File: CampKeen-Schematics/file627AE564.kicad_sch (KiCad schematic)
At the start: 23 parts, among them Q26 2N7000, Q27 2N7000, Q28 2N7000, Q29 2N7000, Q54 LTV-847

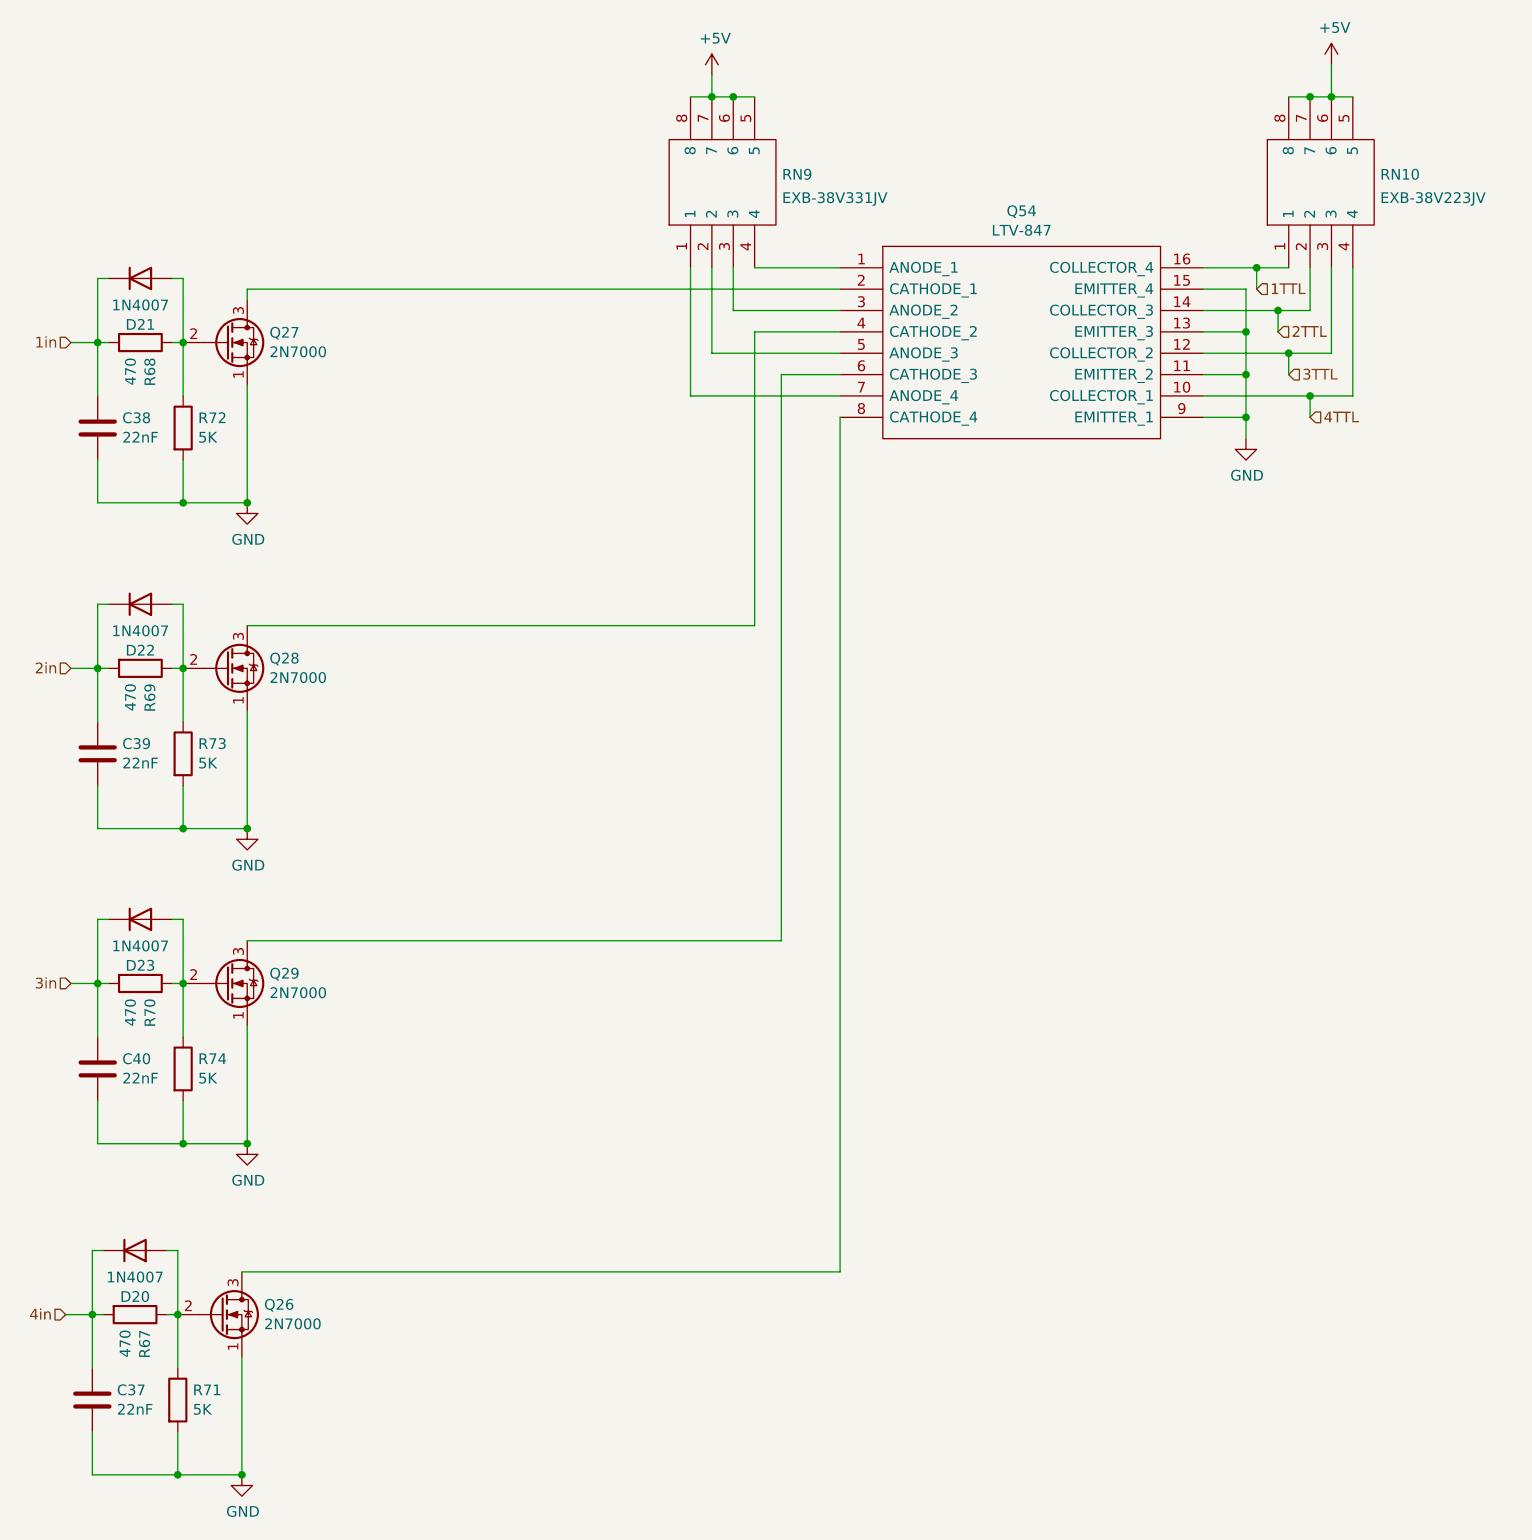
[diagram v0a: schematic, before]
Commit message: working on getting the board cleaned enough to start placing the new designs and chips.
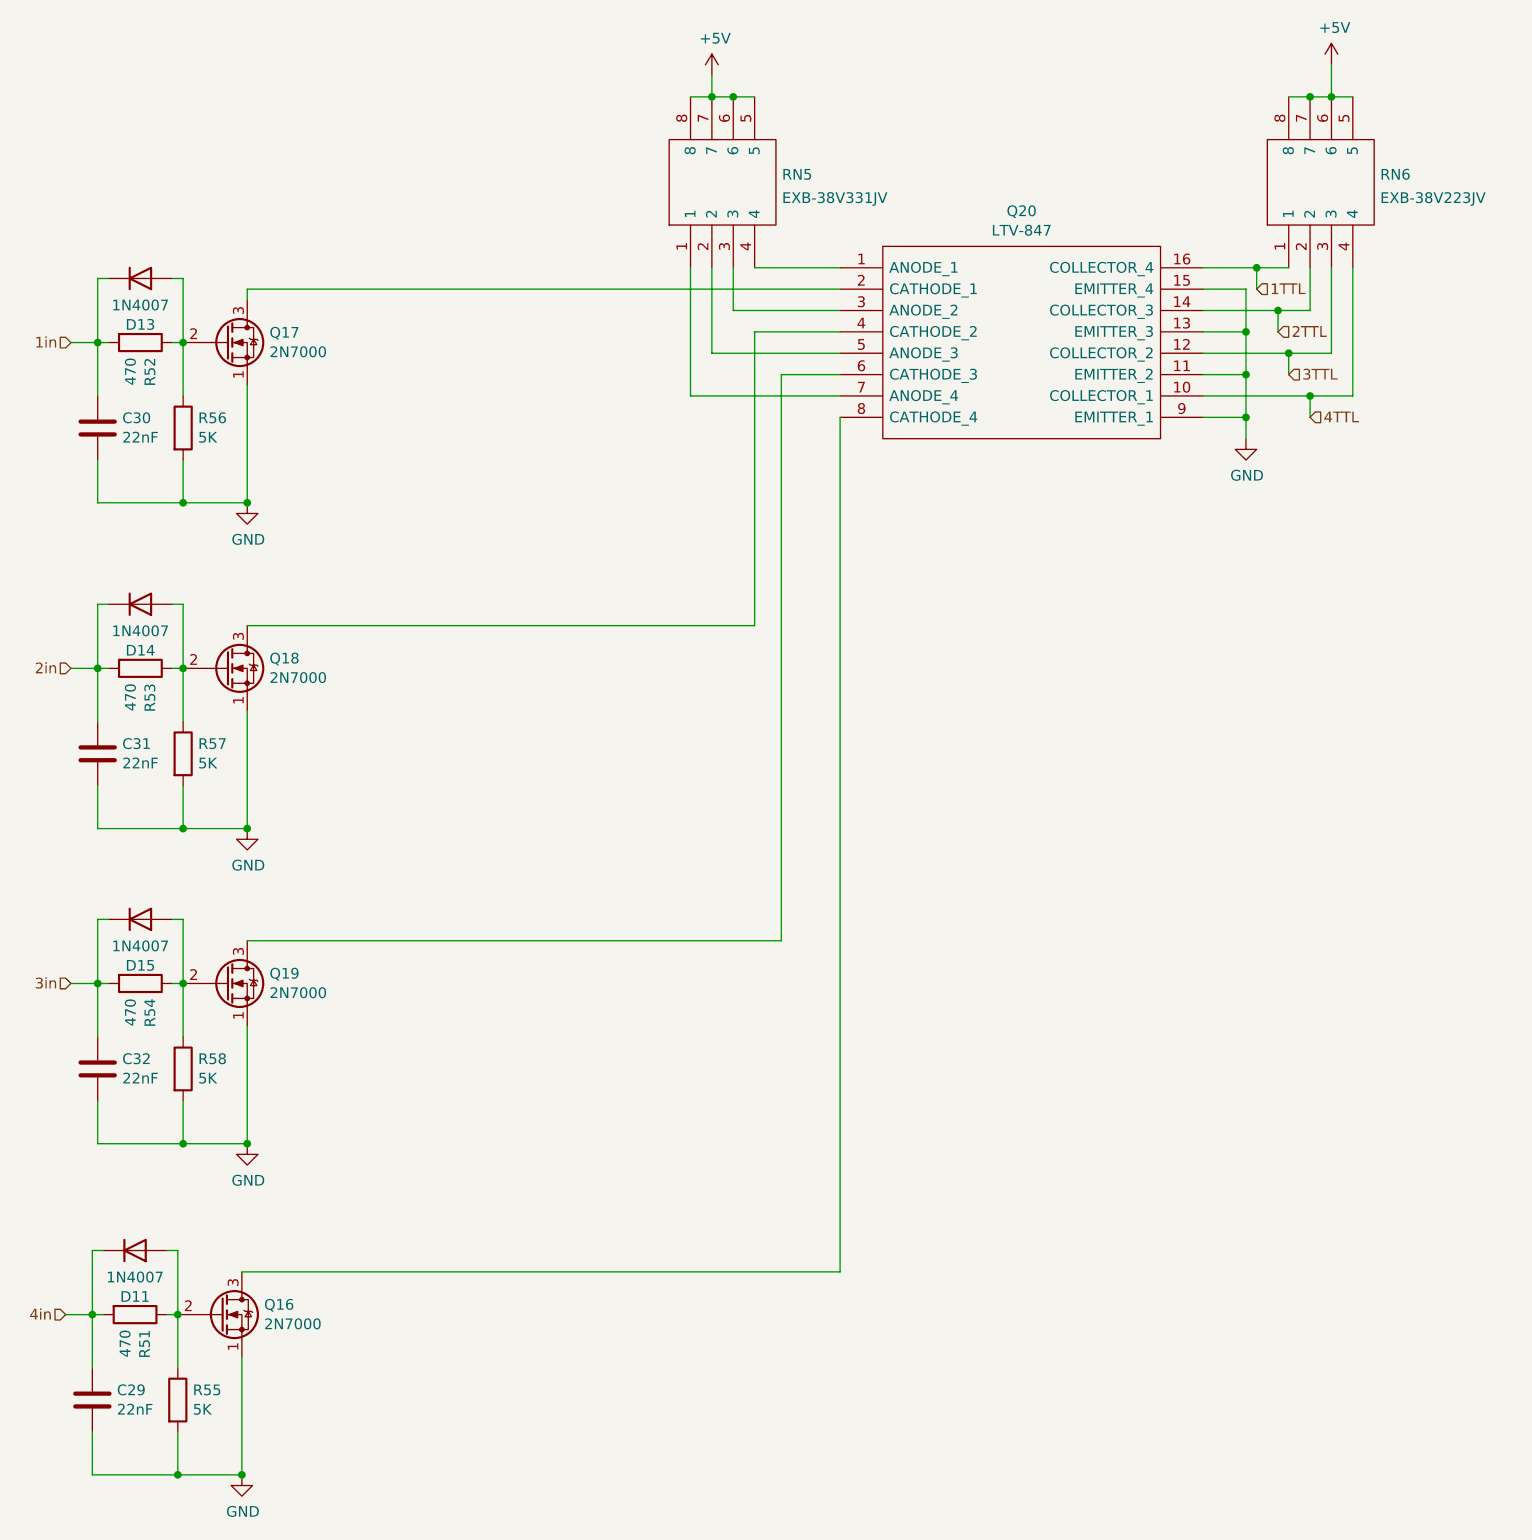
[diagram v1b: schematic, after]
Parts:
- renumbered C37 to C29, C38 to C30, C39 to C31, C40 to C32, D20 to D11, D21 to D13, D22 to D14, D23 to D15, Q26 to Q16, Q27 to Q17, Q28 to Q18, Q29 to Q19, Q54 to Q20, R67 to R51, R68 to R52, R69 to R53, R70 to R54, R71 to R55, R72 to R56, R73 to R57, R74 to R58, RN9 to RN5, RN10 to RN6
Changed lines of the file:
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@@
   (symbol (lib_id "Device:R") (at 67.945 132.08 270)
     (in_bom yes) (on_board yes)
-    (property "Reference" "R70" (id 0) (at 69.1134 133.858 0)
+    (property "Reference" "R54" (id 0) (at 69.1134 133.858 0)
       (effects (font (size 1.27 1.27)) (justify left))
     )
@@
   (symbol (lib_id "Diode:1N4007") (at 67.945 86.995 0) (mirror x)
     (in_bom yes) (on_board yes)
-    (property "Reference" "D22" (id 0) (at 67.945 92.5068 0))
+    (property "Reference" "D14" (id 0) (at 67.945 92.5068 0))
     (property "Value" "1N4007" (id 1) (at 67.945 90.1954 0))
     (property "Footprint" "Diode_THT:D_DO-41_SOD81_P10.16mm_Horizontal" (id 2) (at 67.945 82.55 0)
@@
   (symbol (lib_id "power:+5V") (at 135.89 24.13 0)
     (in_bom yes) (on_board yes)
-    (property "Reference" "#PWR0152" (id 0) (at 135.89 27.94 0)
+    (property "Reference" "#PWR0111" (id 0) (at 135.89 27.94 0)
       (effects (font (size 1.27 1.27)) hide)
     )
@@
   (symbol (lib_id "Samac_Sys:EXB-38V331JV") (at 133.35 46.99 90)
     (in_bom yes) (on_board yes) (fields_autoplaced)
-    (property "Reference" "RN9" (id 0) (at 144.2212 35.9215 90)
+    (property "Reference" "RN5" (id 0) (at 144.2212 35.9215 90)
       (effects (font (size 1.27 1.27)) (justify right))
     )
@@
   (symbol (lib_id "power:GND") (at 80.645 151.13 0)
     (in_bom yes) (on_board yes)
-    (property "Reference" "#PWR0156" (id 0) (at 80.645 157.48 0)
+    (property "Reference" "#PWR0114" (id 0) (at 80.645 157.48 0)
       (effects (font (size 1.27 1.27)) hide)
     )
@@
   (symbol (lib_id "Transistor_FET:2N7000") (at 78.105 55.88 0)
     (in_bom yes) (on_board yes)
-    (property "Reference" "Q27" (id 0) (at 83.2866 54.7116 0)
+    (property "Reference" "Q17" (id 0) (at 83.2866 54.7116 0)
       (effects (font (size 1.27 1.27)) (justify left))
     )
@@
   (symbol (lib_id "Device:R") (at 67.945 55.88 270)
     (in_bom yes) (on_board yes)
-    (property "Reference" "R68" (id 0) (at 69.1134 57.658 0)
+    (property "Reference" "R52" (id 0) (at 69.1134 57.658 0)
       (effects (font (size 1.27 1.27)) (justify left))
     )
@@
   (symbol (lib_id "Diode:1N4007") (at 67.945 124.46 0) (mirror x)
     (in_bom yes) (on_board yes)
-    (property "Reference" "D23" (id 0) (at 67.945 129.9718 0))
+    (property "Reference" "D15" (id 0) (at 67.945 129.9718 0))
     (property "Value" "1N4007" (id 1) (at 67.945 127.6604 0))
     (property "Footprint" "Diode_THT:D_DO-41_SOD81_P10.16mm_Horizontal" (id 2) (at 67.945 120.015 0)
@@
   (symbol (lib_id "power:GND") (at 199.39 67.31 0)
     (in_bom yes) (on_board yes)
-    (property "Reference" "#PWR0155" (id 0) (at 199.39 73.66 0)
+    (property "Reference" "#PWR0113" (id 0) (at 199.39 73.66 0)
       (effects (font (size 1.27 1.27)) hide)
     )
@@
   (symbol (lib_id "SamacSys_Parts:LTV-847") (at 151.13 46.99 0)
     (in_bom yes) (on_board yes)
-    (property "Reference" "Q54" (id 0) (at 172.72 40.259 0))
+    (property "Reference" "Q20" (id 0) (at 172.72 40.259 0))
     (property "Value" "LTV-847" (id 1) (at 172.72 42.5704 0))
     (property "Footprint" "SamacSys_Parts:DIP762W60P254L1984H450Q16N" (id 2) (at 190.5 44.45 0)
@@
   (symbol (lib_id "power:GND") (at 80.645 113.665 0)
     (in_bom yes) (on_board yes)
-    (property "Reference" "#PWR0123" (id 0) (at 80.645 120.015 0)
+    (property "Reference" "#PWR0108" (id 0) (at 80.645 120.015 0)
       (effects (font (size 1.27 1.27)) hide)
     )
@@
   (symbol (lib_id "power:GND") (at 80.01 190.5 0)
     (in_bom yes) (on_board yes)
-    (property "Reference" "#PWR0150" (id 0) (at 80.01 196.85 0)
+    (property "Reference" "#PWR0110" (id 0) (at 80.01 196.85 0)
       (effects (font (size 1.27 1.27)) hide)
     )
@@
   (symbol (lib_id "Device:R") (at 67.945 94.615 270)
     (in_bom yes) (on_board yes)
-    (property "Reference" "R69" (id 0) (at 69.1134 96.393 0)
+    (property "Reference" "R53" (id 0) (at 69.1134 96.393 0)
       (effects (font (size 1.27 1.27)) (justify left))
     )
@@
   (symbol (lib_id "Diode:1N4007") (at 67.31 163.83 0) (mirror x)
     (in_bom yes) (on_board yes)
-    (property "Reference" "D20" (id 0) (at 67.31 169.3418 0))
+    (property "Reference" "D11" (id 0) (at 67.31 169.3418 0))
     (property "Value" "1N4007" (id 1) (at 67.31 167.0304 0))
     (property "Footprint" "Diode_THT:D_DO-41_SOD81_P10.16mm_Horizontal" (id 2) (at 67.31 159.385 0)
@@
   (symbol (lib_id "Device:R") (at 67.31 171.45 270)
     (in_bom yes) (on_board yes)
-    (property "Reference" "R67" (id 0) (at 68.4784 173.228 0)
+    (property "Reference" "R51" (id 0) (at 68.4784 173.228 0)
       (effects (font (size 1.27 1.27)) (justify left))
     )
@@
   (symbol (lib_id "Device:R") (at 73.025 104.775 0)
     (in_bom yes) (on_board yes)
-    (property "Reference" "R73" (id 0) (at 74.803 103.6066 0)
+    (property "Reference" "R57" (id 0) (at 74.803 103.6066 0)
       (effects (font (size 1.27 1.27)) (justify left))
     )
@@
   (symbol (lib_id "Device:R") (at 73.025 142.24 0)
     (in_bom yes) (on_board yes)
-    (property "Reference" "R74" (id 0) (at 74.803 141.0716 0)
+    (property "Reference" "R58" (id 0) (at 74.803 141.0716 0)
       (effects (font (size 1.27 1.27)) (justify left))
     )
@@
   (symbol (lib_id "Transistor_FET:2N7000") (at 77.47 171.45 0)
     (in_bom yes) (on_board yes)
-    (property "Reference" "Q26" (id 0) (at 82.6516 170.2816 0)
+    (property "Reference" "Q16" (id 0) (at 82.6516 170.2816 0)
       (effects (font (size 1.27 1.27)) (justify left))
     )
@@
   (symbol (lib_id "Device:C") (at 62.865 66.04 0)
     (in_bom yes) (on_board yes)
-    (property "Reference" "C38" (id 0) (at 65.786 64.8716 0)
+    (property "Reference" "C30" (id 0) (at 65.786 64.8716 0)
       (effects (font (size 1.27 1.27)) (justify left))
     )
@@
   (symbol (lib_id "power:GND") (at 80.645 74.93 0)
     (in_bom yes) (on_board yes)
-    (property "Reference" "#PWR0124" (id 0) (at 80.645 81.28 0)
+    (property "Reference" "#PWR0109" (id 0) (at 80.645 81.28 0)
       (effects (font (size 1.27 1.27)) hide)
     )
@@
   (symbol (lib_id "Device:R") (at 73.025 66.04 0)
     (in_bom yes) (on_board yes)
-    (property "Reference" "R72" (id 0) (at 74.803 64.8716 0)
+    (property "Reference" "R56" (id 0) (at 74.803 64.8716 0)
       (effects (font (size 1.27 1.27)) (justify left))
     )
@@
   (symbol (lib_id "Device:R") (at 72.39 181.61 0)
     (in_bom yes) (on_board yes)
-    (property "Reference" "R71" (id 0) (at 74.168 180.4416 0)
+    (property "Reference" "R55" (id 0) (at 74.168 180.4416 0)
       (effects (font (size 1.27 1.27)) (justify left))
     )
@@
   (symbol (lib_id "Transistor_FET:2N7000") (at 78.105 132.08 0)
     (in_bom yes) (on_board yes)
-    (property "Reference" "Q29" (id 0) (at 83.2866 130.9116 0)
+    (property "Reference" "Q19" (id 0) (at 83.2866 130.9116 0)
       (effects (font (size 1.27 1.27)) (justify left))
     )
@@
   (symbol (lib_id "Device:C") (at 62.865 104.775 0)
     (in_bom yes) (on_board yes)
-    (property "Reference" "C39" (id 0) (at 65.786 103.6066 0)
+    (property "Reference" "C31" (id 0) (at 65.786 103.6066 0)
       (effects (font (size 1.27 1.27)) (justify left))
     )
@@
   (symbol (lib_id "power:+5V") (at 209.55 22.86 0)
     (in_bom yes) (on_board yes)
-    (property "Reference" "#PWR0153" (id 0) (at 209.55 26.67 0)
+    (property "Reference" "#PWR0112" (id 0) (at 209.55 26.67 0)
       (effects (font (size 1.27 1.27)) hide)
     )
@@
   (symbol (lib_id "Samac_Sys:EXB-38V223JV") (at 204.47 46.99 90)
     (in_bom yes) (on_board yes) (fields_autoplaced)
-    (property "Reference" "RN10" (id 0) (at 215.3412 35.9215 90)
+    (property "Reference" "RN6" (id 0) (at 215.3412 35.9215 90)
       (effects (font (size 1.27 1.27)) (justify right))
     )
@@
   (symbol (lib_id "Transistor_FET:2N7000") (at 78.105 94.615 0)
     (in_bom yes) (on_board yes)
-    (property "Reference" "Q28" (id 0) (at 83.2866 93.4466 0)
+    (property "Reference" "Q18" (id 0) (at 83.2866 93.4466 0)
       (effects (font (size 1.27 1.27)) (justify left))
     )
@@
   (symbol (lib_id "Device:C") (at 62.23 181.61 0)
     (in_bom yes) (on_board yes)
-    (property "Reference" "C37" (id 0) (at 65.151 180.4416 0)
+    (property "Reference" "C29" (id 0) (at 65.151 180.4416 0)
       (effects (font (size 1.27 1.27)) (justify left))
     )
@@
   (symbol (lib_id "Device:C") (at 62.865 142.24 0)
     (in_bom yes) (on_board yes)
-    (property "Reference" "C40" (id 0) (at 65.786 141.0716 0)
+    (property "Reference" "C32" (id 0) (at 65.786 141.0716 0)
       (effects (font (size 1.27 1.27)) (justify left))
     )
@@
   (symbol (lib_id "Diode:1N4007") (at 67.945 48.26 0) (mirror x)
     (in_bom yes) (on_board yes)
-    (property "Reference" "D21" (id 0) (at 67.945 53.7718 0))
+    (property "Reference" "D13" (id 0) (at 67.945 53.7718 0))
     (property "Value" "1N4007" (id 1) (at 67.945 51.4604 0))
     (property "Footprint" "Diode_THT:D_DO-41_SOD81_P10.16mm_Horizontal" (id 2) (at 67.945 43.815 0)
